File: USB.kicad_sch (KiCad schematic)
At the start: 12 parts, among them J1 USB4110GFA, U2 USBLC6-2SC6, U4 TPS2051CDBVR

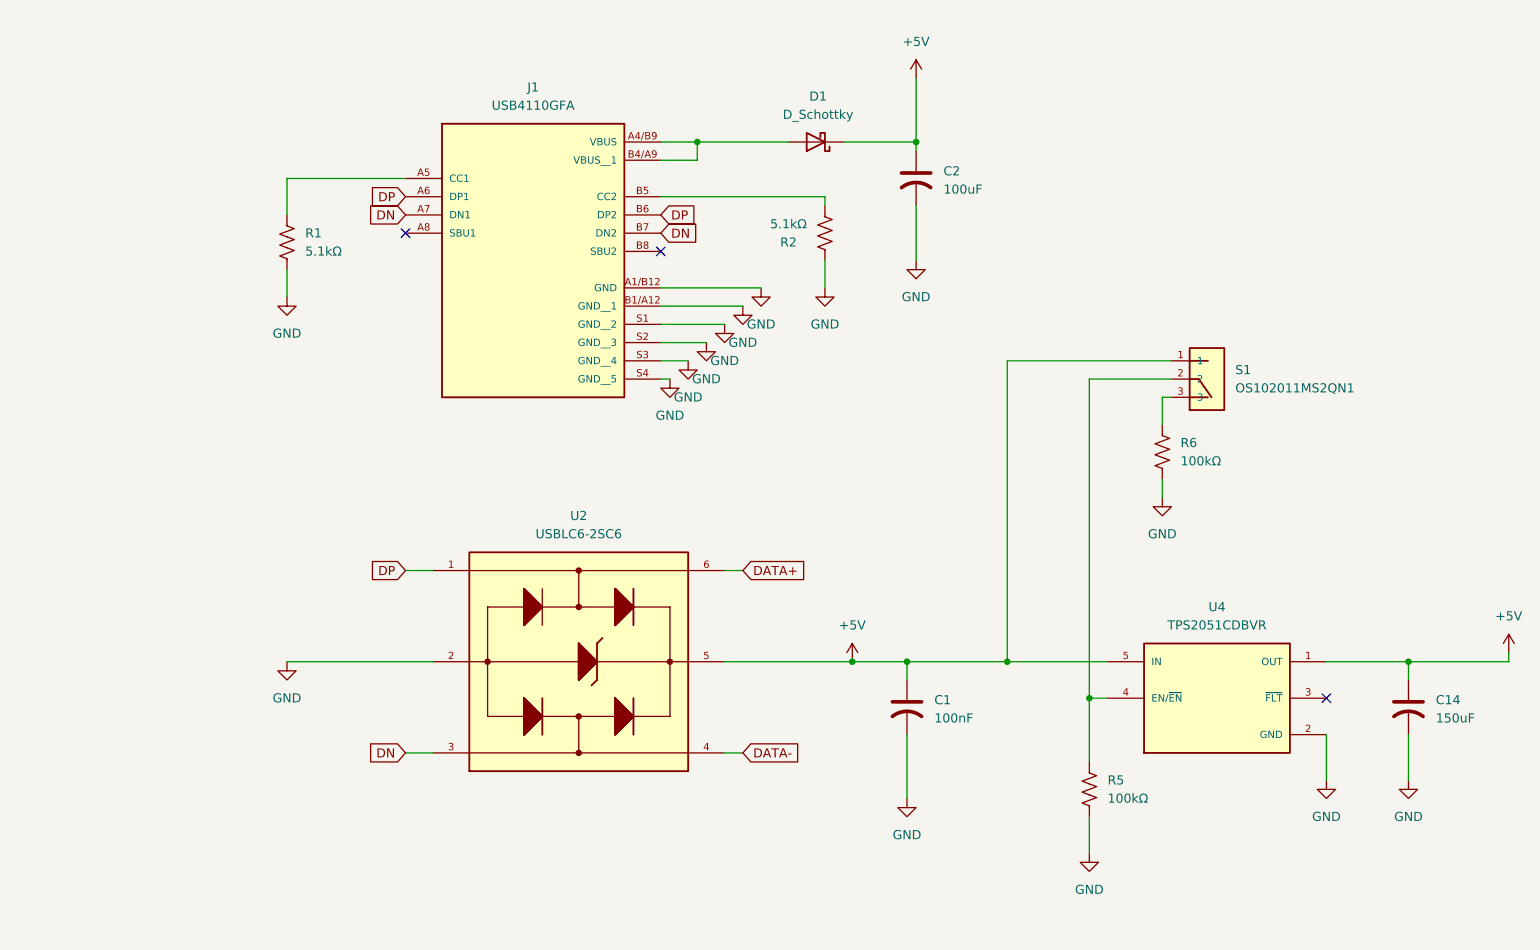
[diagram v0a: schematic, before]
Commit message: Everything is done except for the programming pins
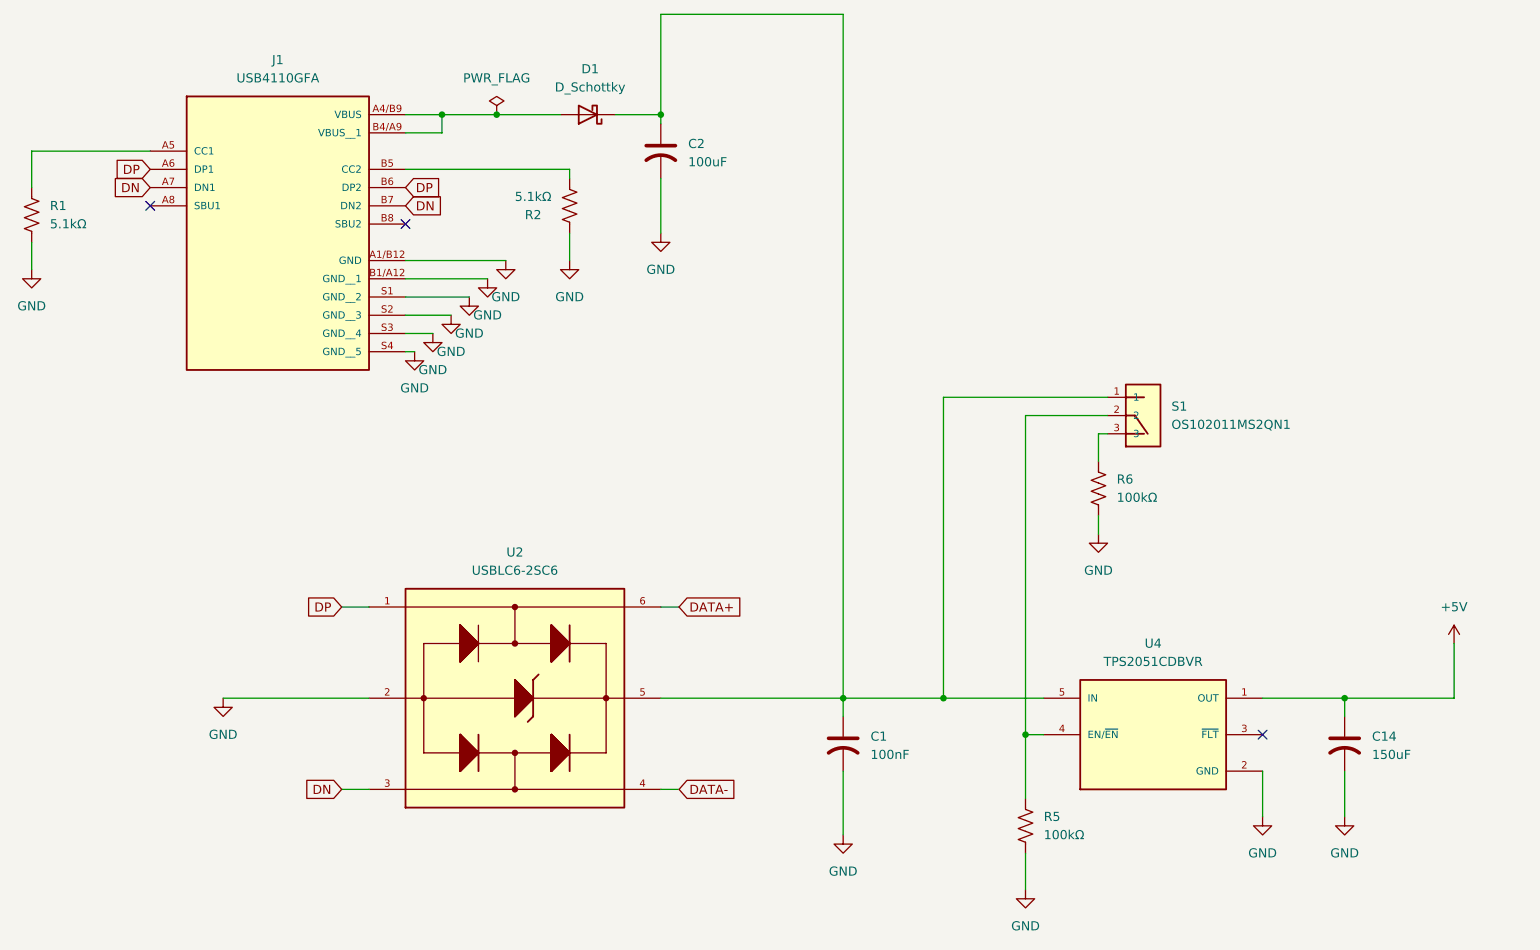
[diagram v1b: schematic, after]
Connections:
- net +5V: no longer C1.1, C2.1, D1.1 (K), S1.1, U2.5, U4.5 (IN)
- new net: C1.1, C2.1, D1.1 (K), S1.1, U2.5, U4.5 (IN)
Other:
- moved on the sheet: C1, C14, C2, D1, J1, R1, R2, R5, R6, S1, U2, U4
